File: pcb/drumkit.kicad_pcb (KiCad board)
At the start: 2 copper layers, 26 parts, among them J1 BATTERY, J2 Conn_01x04_Female, SW1 BUTTON1, SW2 BUTTON2, SW3 BUTTON3, SW4 BUTTON4, SW5 POWER_SW, U1 Pico

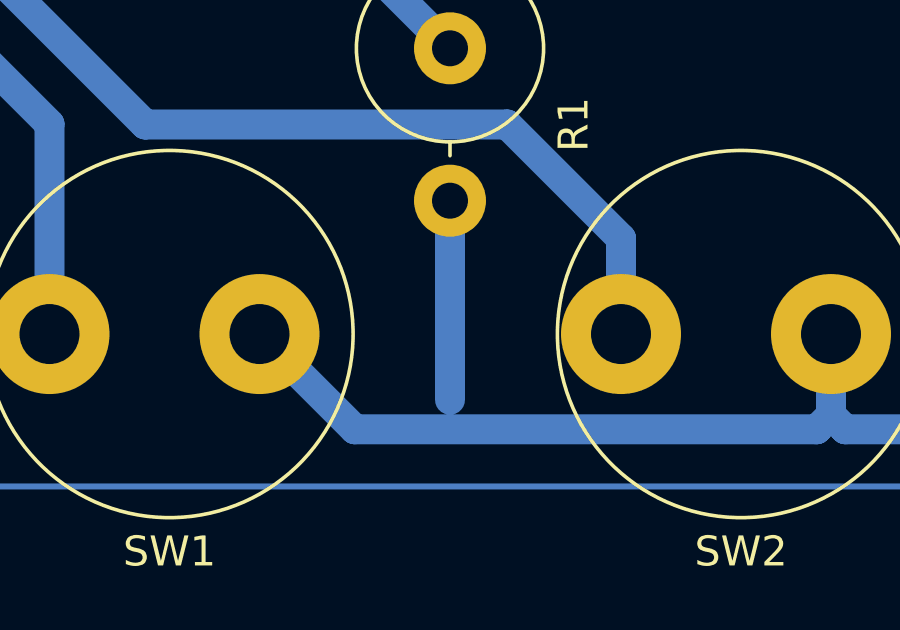
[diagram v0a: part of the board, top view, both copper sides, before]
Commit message: why is it not updating?
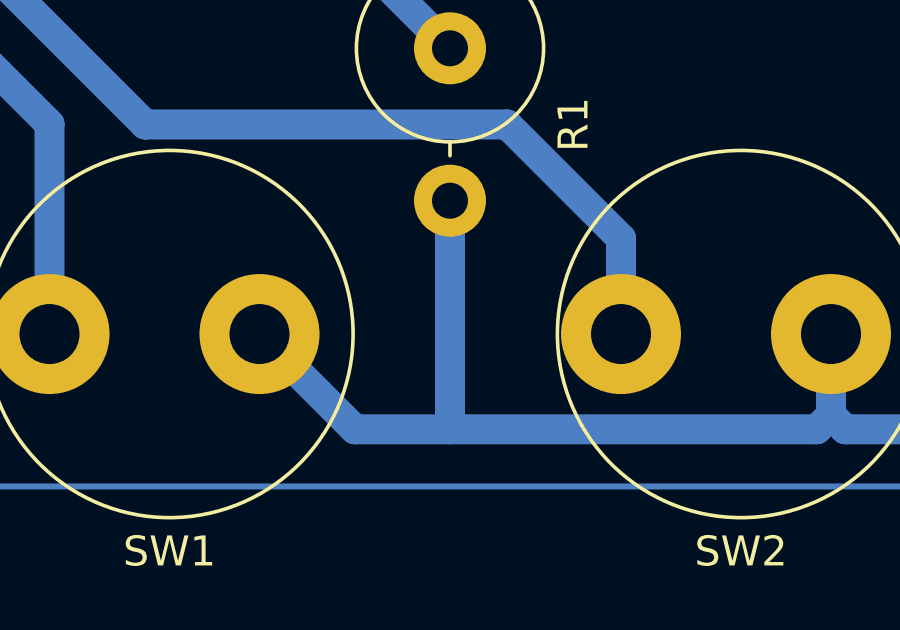
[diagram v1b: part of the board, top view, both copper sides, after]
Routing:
- net GND: track 360.1 -> 361.1 mm
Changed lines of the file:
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@@
   (segment (start 154.265 60.06) (end 154.265 53.716877) (width 2) (layer "B.Cu") (net 8))
   (segment (start 174.625 104.14) (end 174.625 107.155) (width 1) (layer "B.Cu") (net 8))
+  (segment (start 142.875 107.315) (end 142.875 99.695) (width 1) (layer "B.Cu") (net 8))
   (segment (start 176.946877 53.975) (end 177.8 53.121877) (width 2) (layer "B.Cu") (net 8))
-  (segment (start 142.875 99.695) (end 142.875 106.33) (width 1) (layer "B.Cu") (net 8))
   (segment (start 155.575 106.84) (end 156.05 107.315) (width 1) (layer "B.Cu") (net 8))
   (segment (start 160.528 50.927) (end 163.576 53.975) (width 2) (layer "B.Cu") (net 8))
